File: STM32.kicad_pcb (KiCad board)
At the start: 4 copper layers, 38 x 32 mm, 28 parts, among them J1 USB_B_Micro, SW1 SW_SPDT, U1 STM32F103C8Tx, U2 AMS1117-3.3, Y1 Crystal_GND24

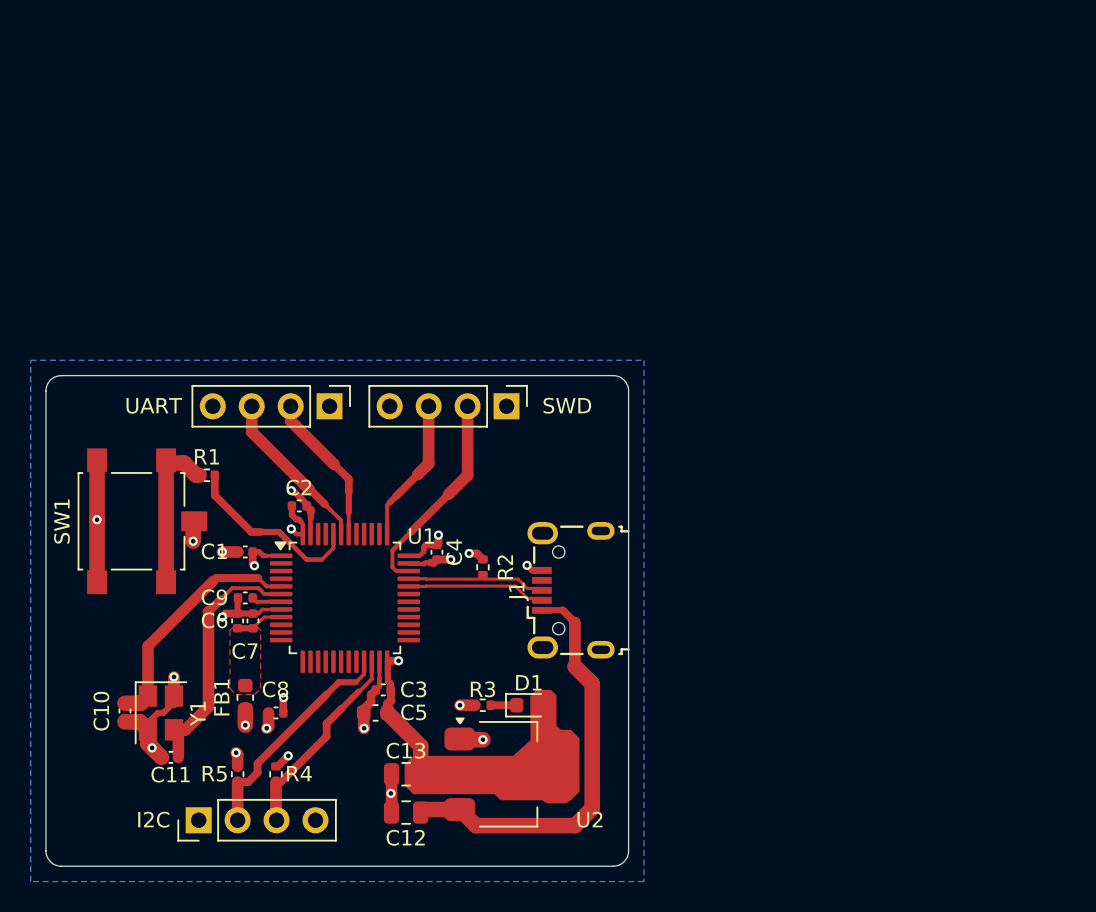
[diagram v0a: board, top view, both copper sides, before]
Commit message: Add files via upload
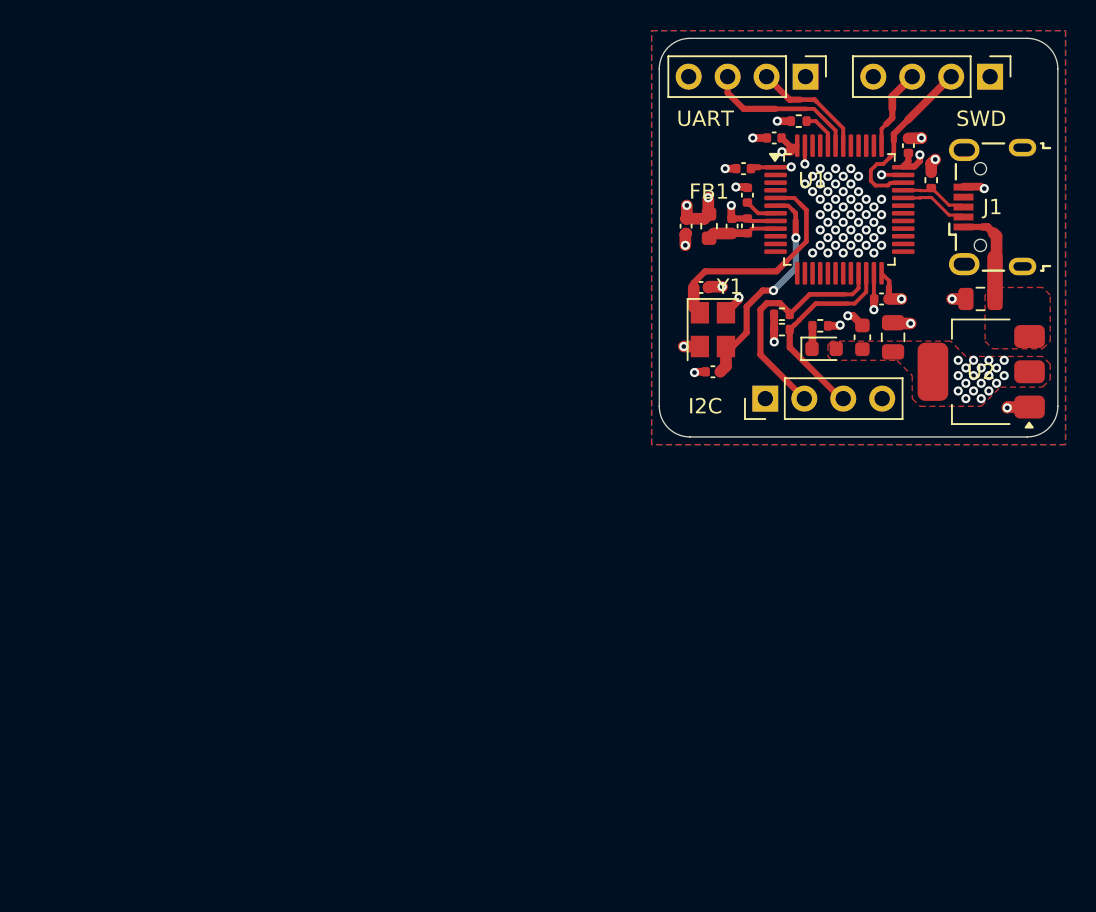
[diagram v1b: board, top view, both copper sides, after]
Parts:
- removed SW1: SW_SPDT, Button_Switch_SMD:SW_SPST_B3S-1100
- moved C12 50.3 mm to (198.9, 80.0)
- moved C10 46.6 mm to (180.7, 79.2), turned to 0 degrees
- moved R5 46.5 mm to (186.0, 81.0), turned to 0 degrees
- moved I2C 46.1 mm to (184.9, 86.5)
- moved R1 45.0 mm to (187.1, 68.4)
- moved R4 43.9 mm to (186.0, 82.0), turned to 0 degrees
- moved Y1 43.8 mm to (181.5, 82.0)
- moved C11 43.4 mm to (181.5, 84.8)
- moved FB1 43.1 mm to (181.2, 75.2), turned to 90 degrees
- moved C13 42.7 mm to (193.2, 82.5), turned to 90 degrees
- moved C9 42.0 mm to (183.8, 73.2), turned to 90 degrees
- moved C8 41.5 mm to (179.8, 75.2), turned to -90 degrees
- moved C3 41.3 mm to (192.5, 80.0)
- moved C7 41.3 mm to (183.8, 75.2)
- moved C6 41.3 mm to (182.8, 75.2)
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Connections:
- R1 pad 1: /SW_BOOT0 -> GND
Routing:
- net VBUS: track 27.2 -> 6.54 mm
- net GND: track 40.6 -> 24.9 mm, vias 13 -> 72
- net /SW_BOOT0: track 10.5 -> 0.00 mm
- net /BOOT0: track 12.0 -> 2.53 mm
- net +3.3V: track 24.6 -> 16.8 mm, vias 10 -> 27
- net /USB_D-: track 9.08 -> 4.47 mm
- net /USB_D+: track 9.00 -> 4.39 mm
- net /SWCLK: track 9.46 -> 5.33 mm
- net /USART1_TX: track 9.91 -> 7.53 mm
- net /SWDIO: track 13.7 -> 11.5 mm
- net /HSE_OUT: track 16.5 -> 14.6 mm, vias 0 -> 2
- net /USART1_RX: track 11.9 -> 10.1 mm
- net +3.3VA: track 3.14 -> 4.60 mm
- net /HSE_IN: track 15.7 -> 15.0 mm
- net /I2C2_SCL: track 14.9 -> 15.6 mm
- added copper zone on F.Cu, net +3.3V
- added copper zone on F.Cu, net GND
- added copper zone on F.Cu, net VBUS
- removed copper zone on F.Cu, net +3.3VA
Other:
- board size 38 x 32 mm -> 26 x 26 mm
